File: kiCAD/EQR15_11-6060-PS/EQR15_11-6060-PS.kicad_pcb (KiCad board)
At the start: 2 copper layers, 14 x 14 mm, 17 parts, among them J1 Conn, J2 Conn, J3 Conn, J4 Conn, J5 Conn

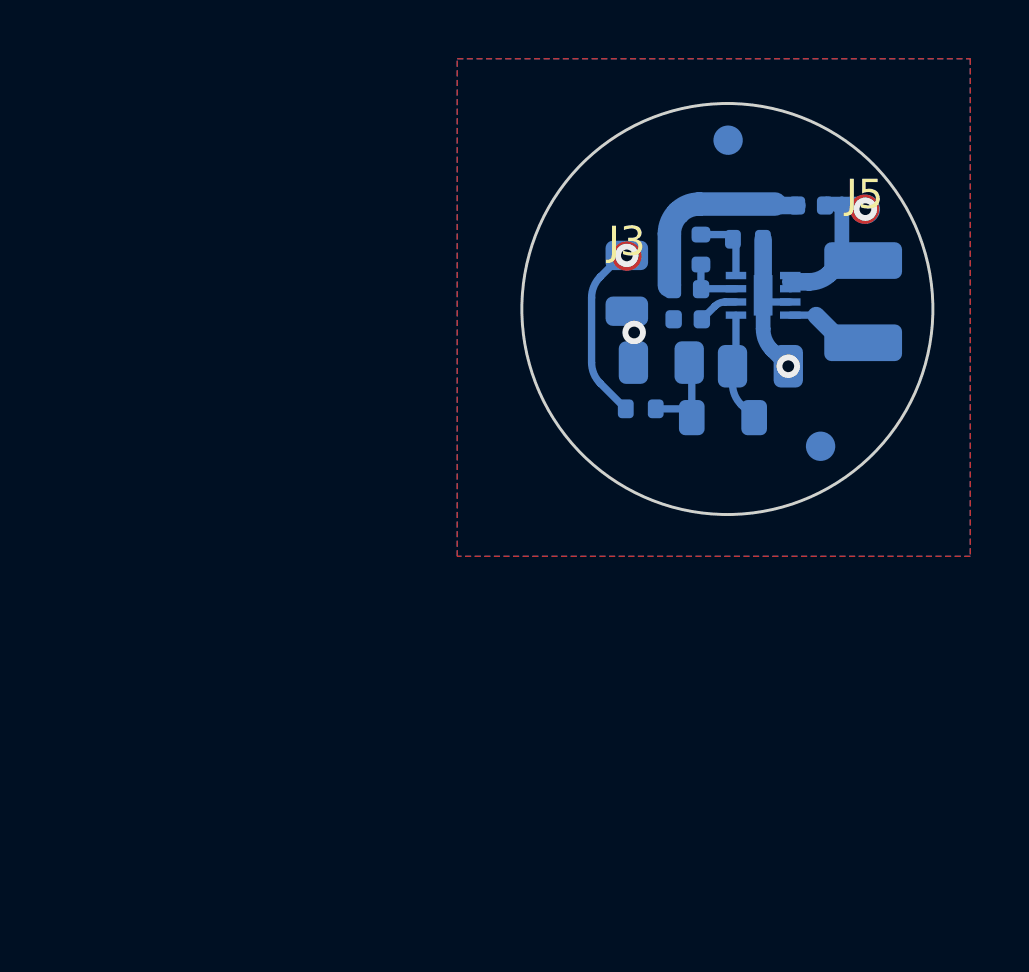
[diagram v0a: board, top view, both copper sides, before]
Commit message: новый файл:    Documents/DoZer-current.png 	новый файл:    Documents/LT8410-current.png 	изменено:      kiCAD/EQR15_11-6060-PS/EQR15_11-6060-PS.kicad_pcb 	изменено:      kiCAD/EQR15_11-6060-PS/EQR15_11-6060-PS.kicad_sch
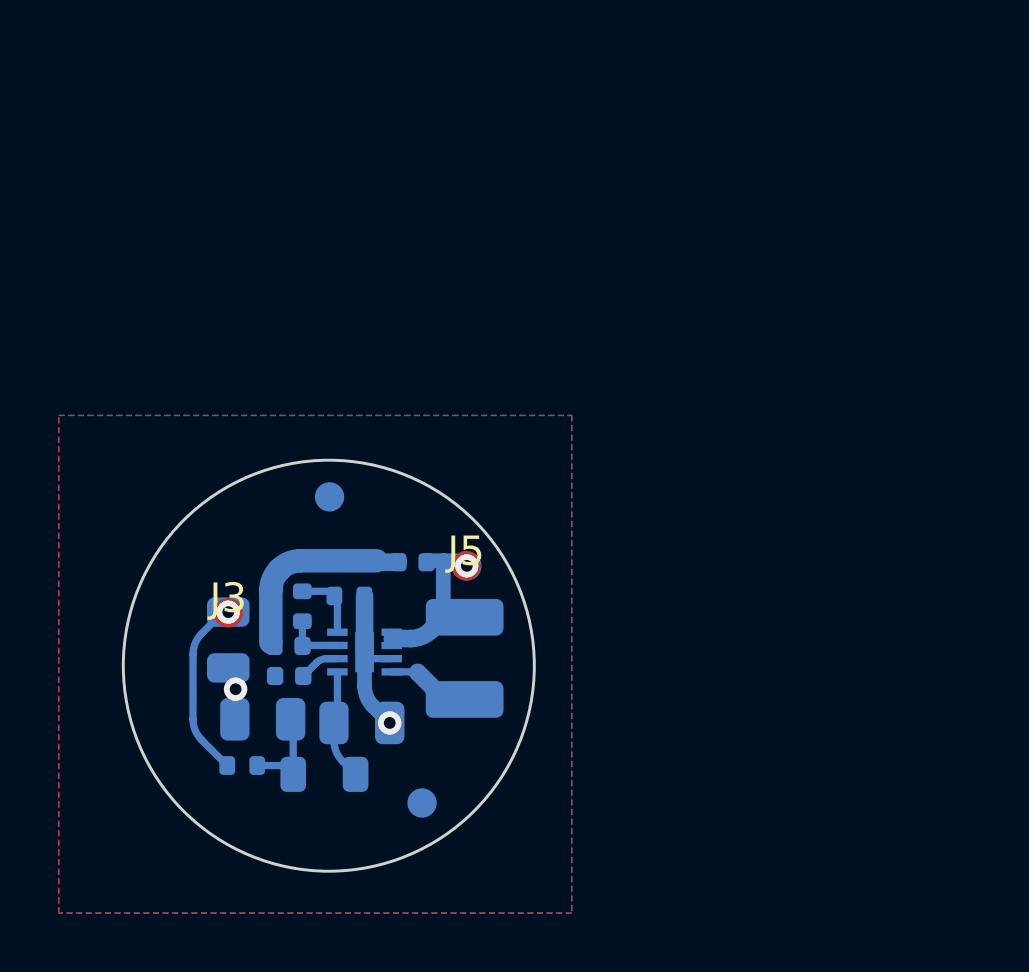
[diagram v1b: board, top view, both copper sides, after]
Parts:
- C3: value 10u -> .1
- moved J3 18.2 mm to (38.4, 49.6)
- moved L2 18.2 mm to (41.7, 55.1)
- moved C1 18.2 mm to (44.7, 47.9)
- moved C3 18.2 mm to (40.5, 50.7)
- moved C4 18.2 mm to (43.0, 53.3)
- moved C5 18.2 mm to (39.6, 53.2)
- moved C6 18.2 mm to (38.4, 50.5)
- moved D1 18.2 mm to (43.0, 50.9)
- moved J1 18.2 mm to (46.5, 48.0)
- moved J4 18.2 mm to (45.0, 56.0)
- moved J5 18.2 mm to (46.5, 48.0)
- moved R1 18.2 mm to (42.5, 49.0)
- moved R2 18.2 mm to (40.9, 49.4)
- moved R3 18.2 mm to (38.9, 54.8)
- moved C2 18.2 mm to (40.5, 51.7)
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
